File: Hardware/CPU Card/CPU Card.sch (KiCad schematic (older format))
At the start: 9 parts, among them IC1 W65C02S6TPG-14, J1 Conn_02x02_Odd_Even

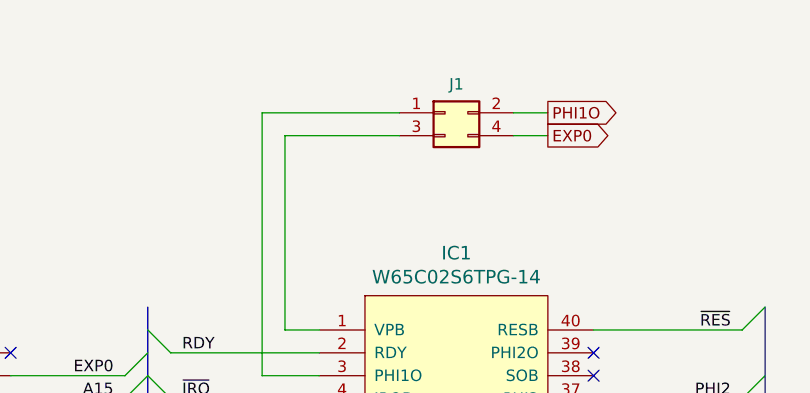
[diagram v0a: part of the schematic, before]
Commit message: Layout CPU card
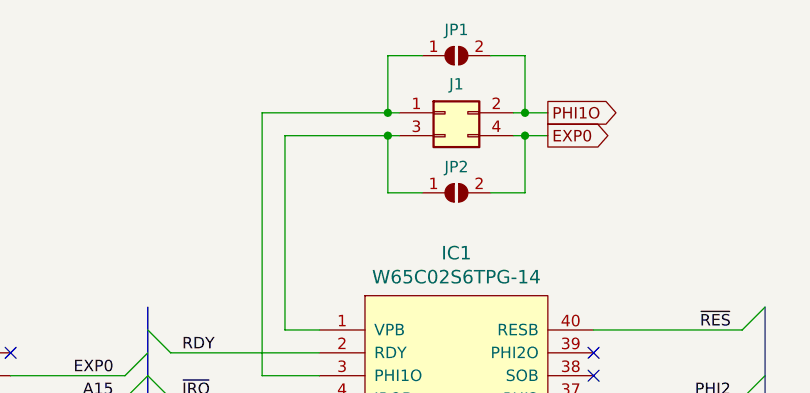
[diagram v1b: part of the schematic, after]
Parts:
- added JP1, JP2: SolderJumper_2_Open, Jumper:SolderJumper-2_P1.3mm_Open_RoundedPad1.0x1.5mm, symbol Jumper:SolderJumper_2_Open
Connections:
- net EXP0: now also JP2.2 (B)
- net PHI1O: now also JP1.2 (B)
- net at IC1.1 (VPB), J1.3 (Pin_3): now also JP2.1 (A)
- net at IC1.3 (PHI1O), J1.1 (Pin_1): now also JP1.1 (A)
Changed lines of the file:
@@
 	4800 2750 4800 1900
 Wire Wire Line
-	4800 1900 5300 1900
+	4800 1900 5250 1900
 Wire Wire Line
 	4950 2950 4700 2950
@@
 	4700 2950 4700 1800
 Wire Wire Line
-	4700 1800 5300 1800
-Wire Wire Line
-	5800 1800 5950 1800
-Wire Wire Line
-	5800 1900 5950 1900
+	4700 1800 5250 1800
+Wire Wire Line
+	5800 1800 5850 1800
+Wire Wire Line
+	5800 1900 5850 1900
 Text GLabel 5950 1900 2    50   Output ~ 0
 EXP0
@@
 Wire Wire Line
 	8400 4600 8400 4750
+$Comp
+L Jumper:SolderJumper_2_Open JP2
+U 1 1 606F23BA
+P 5550 2150
+F 0 "JP2" H 5550 2263 50  0000 C CNN
+F 1 "SolderJumper_2_Open" H 5550 2264 50  0001 C CNN
+F 2 "Jumper:SolderJumper-2_P1.3mm_Open_RoundedPad1.0x1.5mm" H 5550 2150 50  0001 C CNN
+F 3 "~" H 5550 2150 50  0001 C CNN
+	1    5550 2150
+	1    0    0    -1
+$EndComp
+$Comp
+L Jumper:SolderJumper_2_Open JP1
+U 1 1 606F2C26
+P 5550 1550
+F 0 "JP1" H 5550 1663 50  0000 C CNN
+F 1 "SolderJumper_2_Open" H 5550 1664 50  0001 C CNN
+F 2 "Jumper:SolderJumper-2_P1.3mm_Open_RoundedPad1.0x1.5mm" H 5550 1550 50  0001 C CNN
+F 3 "~" H 5550 1550 50  0001 C CNN
+	1    5550 1550
+	1    0    0    -1
+$EndComp
+Wire Wire Line
+	5700 1550 5850 1550
+Wire Wire Line
+	5850 1550 5850 1800
+Connection ~ 5850 1800
+Wire Wire Line
+	5850 1800 5950 1800
+Wire Wire Line
+	5400 1550 5250 1550
+Wire Wire Line
+	5250 1550 5250 1800
+Connection ~ 5250 1800
+Wire Wire Line
+	5250 1800 5300 1800
+Wire Wire Line
+	5400 2150 5250 2150
+Wire Wire Line
+	5250 2150 5250 1900
+Connection ~ 5250 1900
+Wire Wire Line
+	5250 1900 5300 1900
+Wire Wire Line
+	5700 2150 5850 2150
+Wire Wire Line
+	5850 2150 5850 1900
 Wire Bus Line
 	4200 2650 4200 5300
@@
 Wire Bus Line
 	1800 2650 1800 5300
+Connection ~ 5850 1900
+Wire Wire Line
+	5850 1900 5950 1900
 $EndSCHEMATC

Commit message: Generate production files
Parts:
- C1: LCSC (none) -> C49678
- R1, R2, R3, R4, R5: LCSC (none) -> C17513
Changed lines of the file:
@@
 F 2 "Resistor_SMD:R_0805_2012Metric" V 8730 2850 50  0001 C CNN
 F 3 "~" H 8800 2850 50  0001 C CNN
+F 4 "C17513" H 8800 2850 50  0001 C CNN "LCSC"
 	1    8800 2850
 	0    1    1    0
@@
 F 2 "Resistor_SMD:R_0805_2012Metric" V 8730 3150 50  0001 C CNN
 F 3 "~" H 8800 3150 50  0001 C CNN
+F 4 "C17513" H 8800 3150 50  0001 C CNN "LCSC"
 	1    8800 3150
 	0    1    1    0
@@
 F 2 "Resistor_SMD:R_0805_2012Metric" V 8730 3450 50  0001 C CNN
 F 3 "~" H 8800 3450 50  0001 C CNN
+F 4 "C17513" H 8800 3450 50  0001 C CNN "LCSC"
 	1    8800 3450
 	0    1    1    0
@@
 F 2 "Resistor_SMD:R_0805_2012Metric" V 8730 3750 50  0001 C CNN
 F 3 "~" H 8800 3750 50  0001 C CNN
+F 4 "C17513" H 8800 3750 50  0001 C CNN "LCSC"
 	1    8800 3750
 	0    1    1    0
@@
 F 2 "Resistor_SMD:R_0805_2012Metric" V 8730 4050 50  0001 C CNN
 F 3 "~" H 8800 4050 50  0001 C CNN
+F 4 "C17513" H 8800 4050 50  0001 C CNN "LCSC"
 	1    8800 4050
 	0    1    1    0
@@
 F 2 "Capacitor_SMD:C_0805_2012Metric" H 8438 4200 50  0001 C CNN
 F 3 "~" H 8400 4350 50  0001 C CNN
+F 4 "C49678" H 8400 4350 50  0001 C CNN "LCSC"
 	1    8400 4350
 	1    0    0    -1
@@
 Wire Wire Line
 	5850 2150 5850 1900
+Connection ~ 5850 1900
+Wire Wire Line
+	5850 1900 5950 1900
 Wire Bus Line
 	4200 2650 4200 5300
@@
 Wire Bus Line
 	1800 2650 1800 5300
-Connection ~ 5850 1900
-Wire Wire Line
-	5850 1900 5950 1900
 $EndSCHEMATC
